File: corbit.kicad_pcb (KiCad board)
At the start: 2 copper layers, 6.1 x 13.9 mm, 44 parts, among them J1 Conn_01x02, SW1 SW_Push, SW10 SW_Push, SW11 SW_Push, SW12 SW_Push, SW13 SW_Push, SW14 SW_Push, SW15 SW_Push, SW16 SW_Push, SW17 SW_Push, SW18 SW_Push, SW19 SW_Push, SW2 SW_Push, SW20 SW_Push, SW21 RotaryEncoder, SW22 SW_SPDT, SW3 SW_Push, SW4 SW_Push, SW5 SW_Push, SW6 SW_Push, SW7 SW_Push, SW8 SW_Push, SW9 SW_Push, U1 XIAO-nRF52840-Plus-SMD

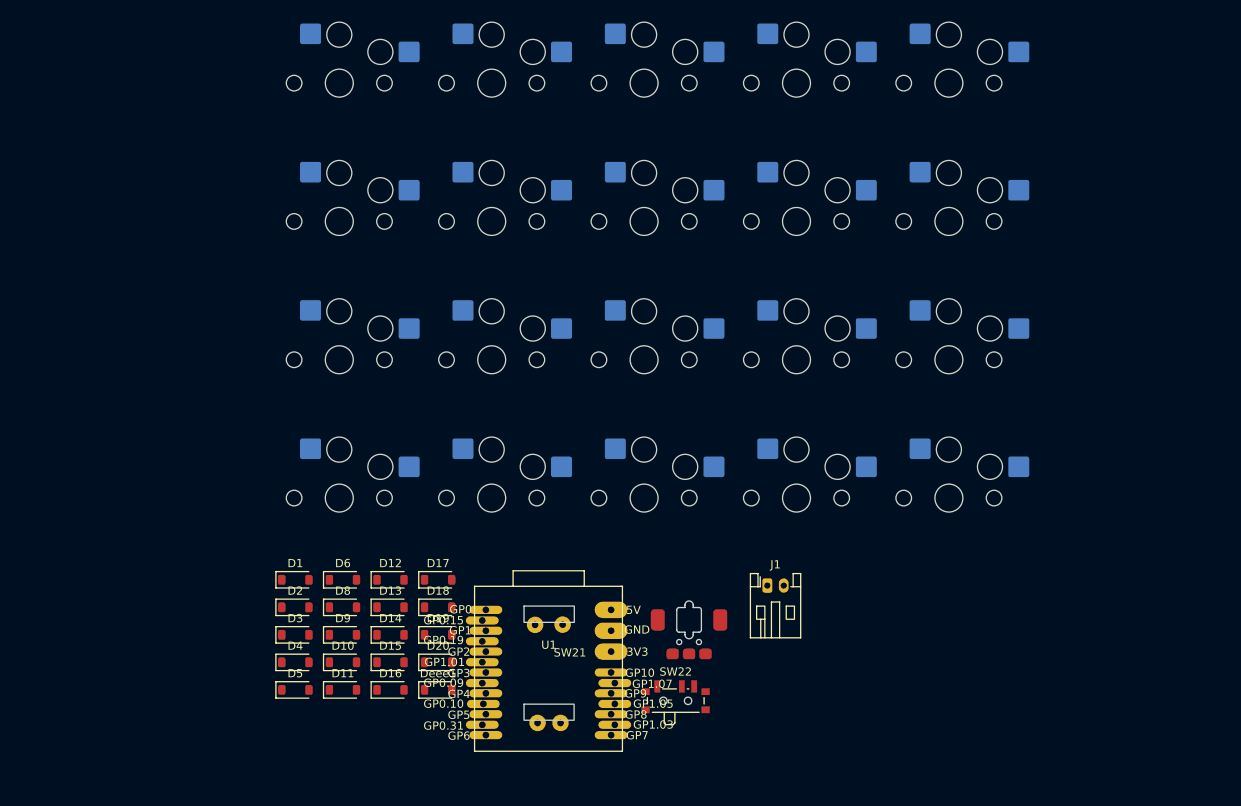
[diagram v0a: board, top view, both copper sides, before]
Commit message: edit pcb
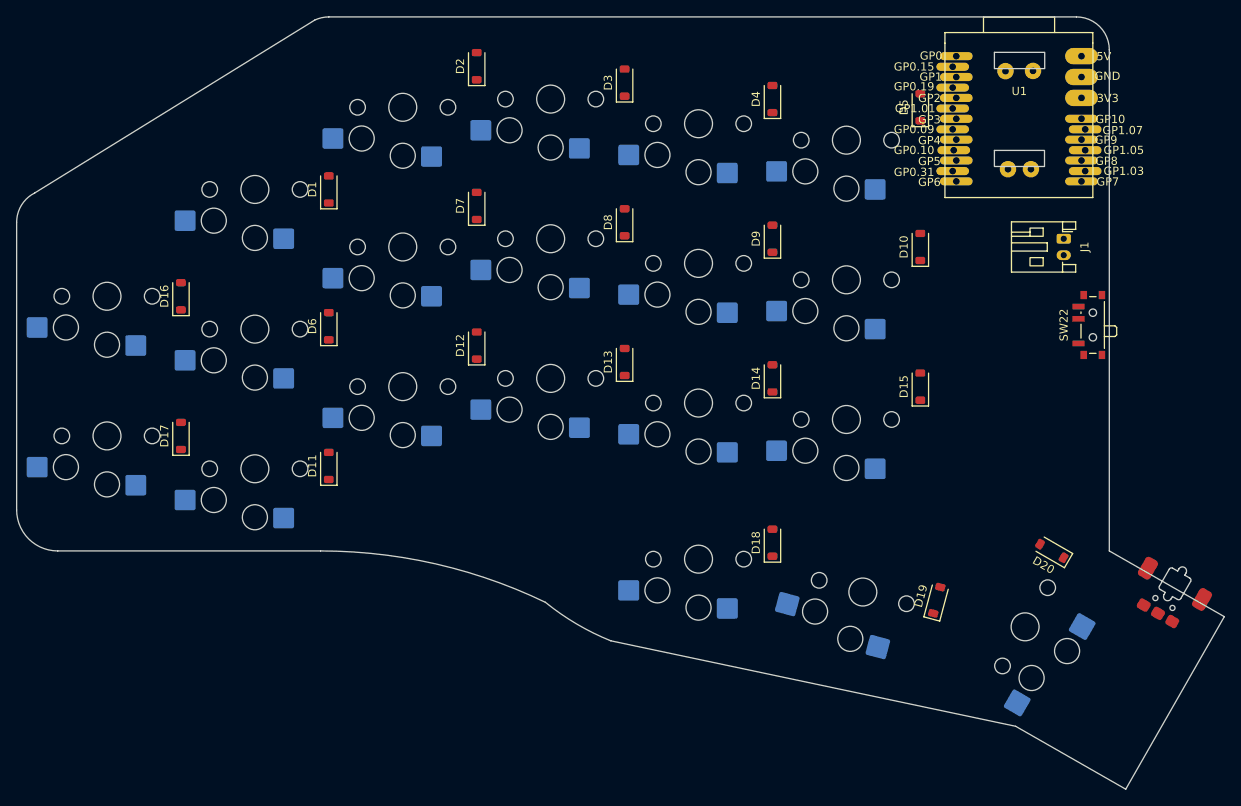
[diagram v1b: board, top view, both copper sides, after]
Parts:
- moved SW17 111.1 mm to (61.0, 113.0), turned to 180 degrees
- moved D5 104.0 mm to (160.0, 73.0), turned to 90 degrees
- moved D4 89.9 mm to (142.0, 72.0), turned to 90 degrees
- moved U1 88.4 mm to (172.1, 71.0)
- moved SW16 87.4 mm to (61.0, 96.0), turned to 180 degrees
- moved D10 86.6 mm to (160.0, 90.0), turned to 90 degrees
- moved D3 78.3 mm to (124.0, 70.0), turned to 90 degrees
- moved D20 75.9 mm to (176.0, 127.0), turned to 150 degrees
- moved D15 72.7 mm to (160.0, 107.0), turned to 90 degrees
- moved D9 71.1 mm to (142.0, 89.0), turned to 90 degrees
- moved D2 69.5 mm to (106.0, 68.0), turned to 90 degrees
- moved SW22 67.9 mm to (180.7, 99.5), turned to 90 degrees
- moved SW4 63.2 mm to (133.0, 75.0), turned to 180 degrees
- moved D19 60.8 mm to (162.0, 133.0), turned to 75 degrees
- moved SW21 59.3 mm to (191.0, 131.0), turned to -30 degrees
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- renumbered Deee1 to D7
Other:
- board size 6.1 x 13.9 mm -> 147 x 94 mm
